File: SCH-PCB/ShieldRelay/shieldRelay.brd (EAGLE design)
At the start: 99.1 x 84.1 mm, 66 parts, among them IC1 LM2596SX-5.0_NOPB, IC2 LM1117MPX-33NOPB, K1 SLA-05VDC-SL-C, K2 SRD-05VDC-SL-C, K3 G3MB-202PL-DC5, K5 G3MB-202PL-DC5, K6 SRD-05VDC-SL-C, Q1 MMST2222A-7-F, Q2 MMST2222A-7-F, Q3 MMST2222A-7-F, Q4 MMST2222A-7-F, Q5 MMST2222A-7-F

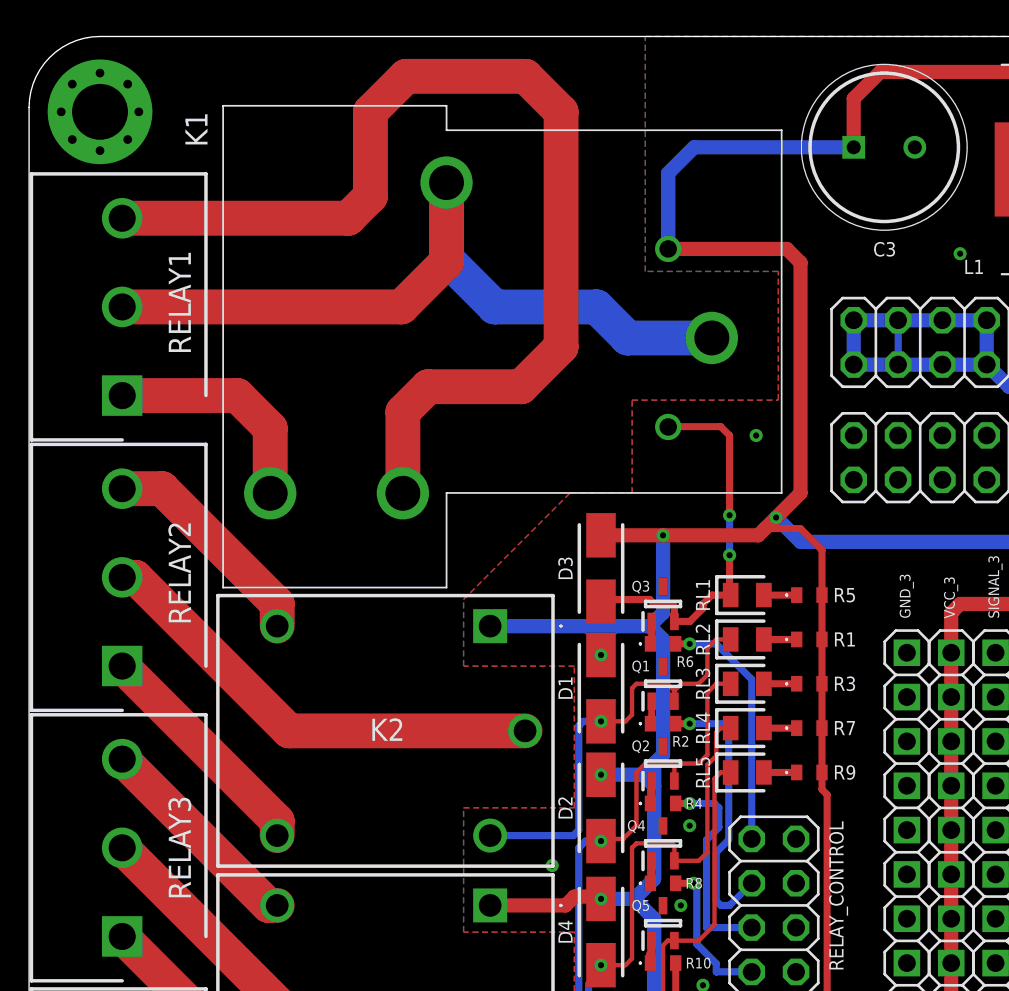
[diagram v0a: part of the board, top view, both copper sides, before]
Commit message: FEAT: add 3D model
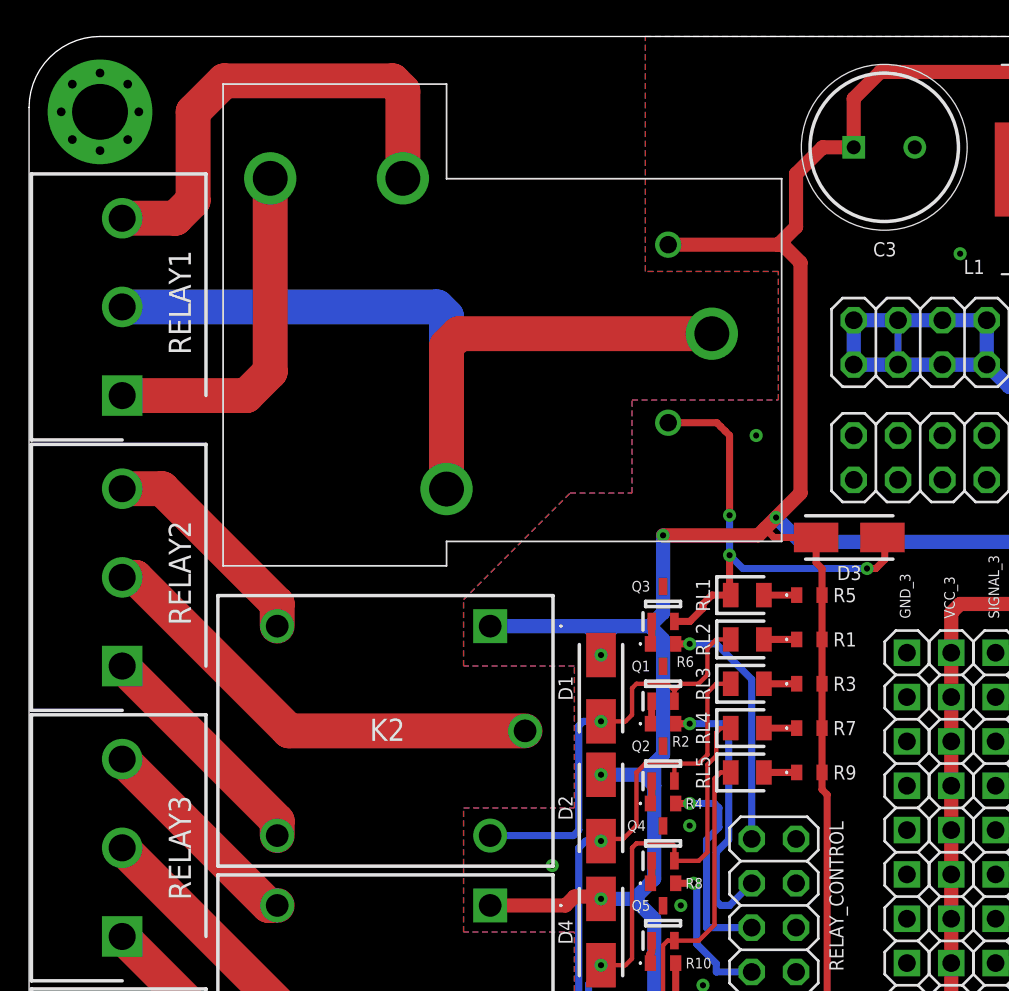
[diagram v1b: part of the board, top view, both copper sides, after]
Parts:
- moved D3 14.3 mm to (47.0, 71.4), turned to 0 degrees
- moved K1 0.24 mm to (39.1, 83.0), flipped to the bottom, turned to 270 degrees
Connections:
- net +5V: now also K1.6; no longer K1.5
- net N$8: now also K1.5; no longer K1.6
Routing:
- net NO2: track 60.9 -> 27.6 mm
- net +5V: track 312.8 -> 302.4 mm
- net NC2: track 13.0 -> 20.1 mm
- net COM2: track 45.6 -> 52.4 mm
- net N$8: track 22.2 -> 28.0 mm, vias 2 -> 3
